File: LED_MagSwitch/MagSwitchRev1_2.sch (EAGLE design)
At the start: 11 parts, among them X1 SWT1, X2 MSTBA4

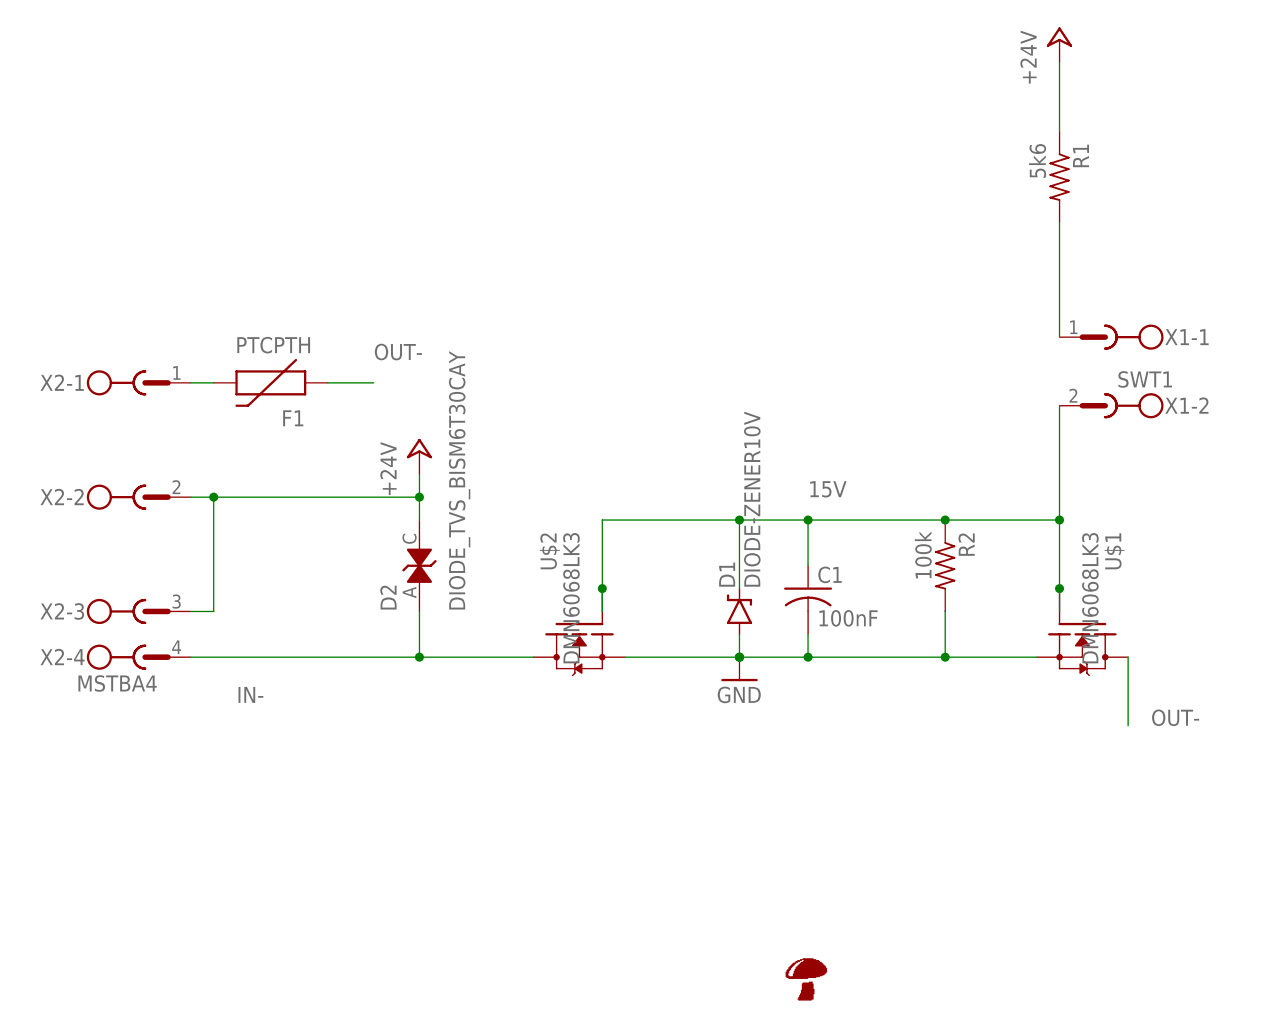
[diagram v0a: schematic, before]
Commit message: CameraSliderFirmware dev
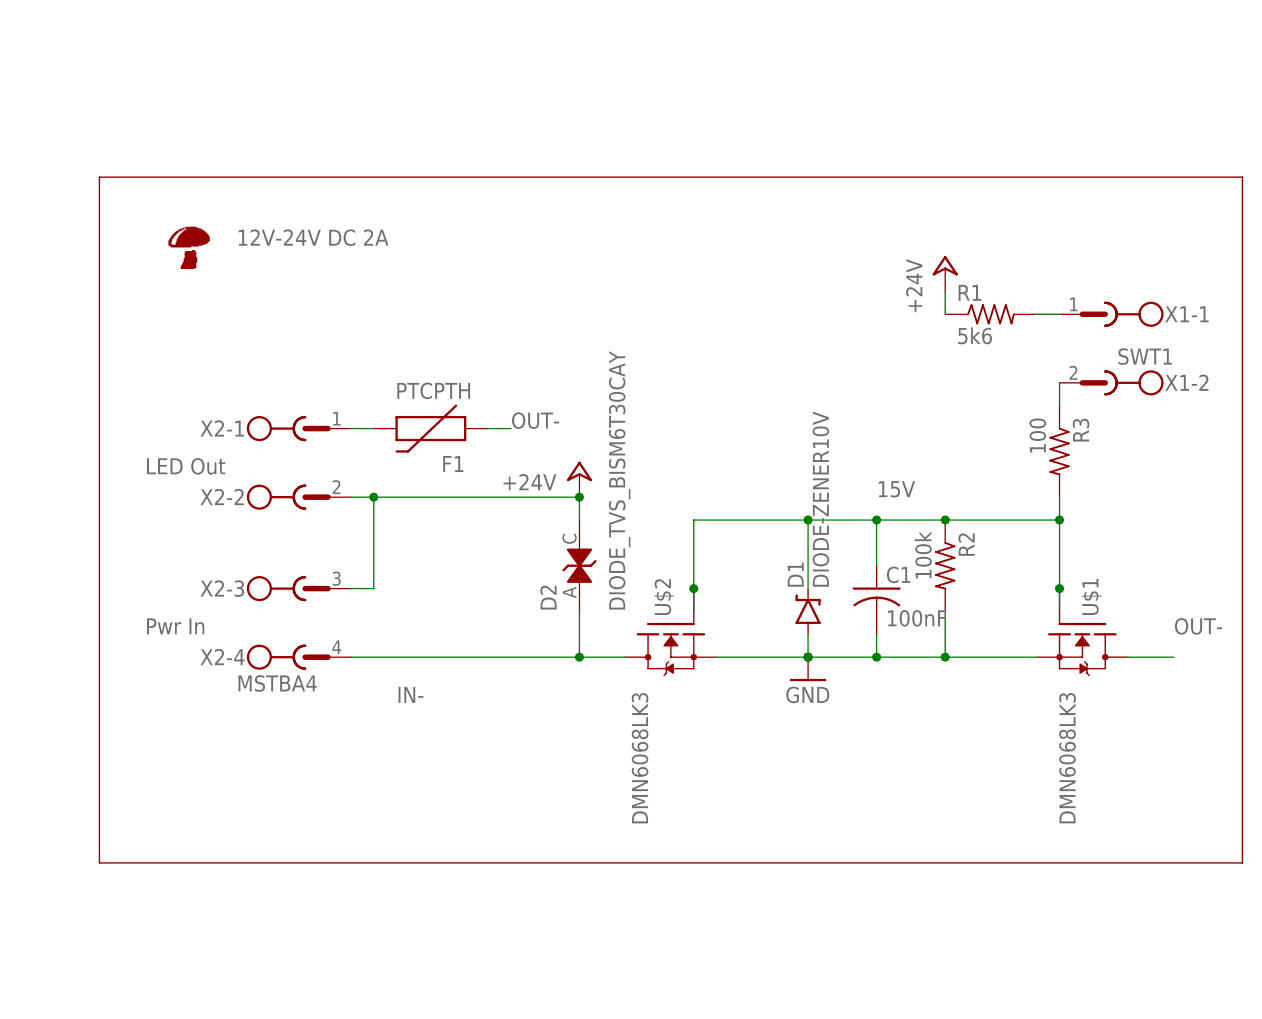
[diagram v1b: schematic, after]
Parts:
- added R3: 100, resistor:R-US_M0805
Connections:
- new net N$3: R3.1, X1-2.1
- net 15V: now also R3.2; no longer X1-2.1
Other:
- note added: "12V-24V DC 2A"
- note added: "LED Out"
- note added: "Pwr In"
- moved on the sheet: C1, D1, D2, F1, R1, U$2, X1-1, X1-2, X2-1, X2-2, X2-3, X2-4
